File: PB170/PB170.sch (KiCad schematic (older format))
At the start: 50 parts, among them J1 USB_C_Receptacle_USB2.0-Conne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, J2 USB_B_Micro, Q1 P-MOSFET-MLP_HS, Q2 BC817, SW1 SW_MEC_5E, SW2 SW_MEC_5E

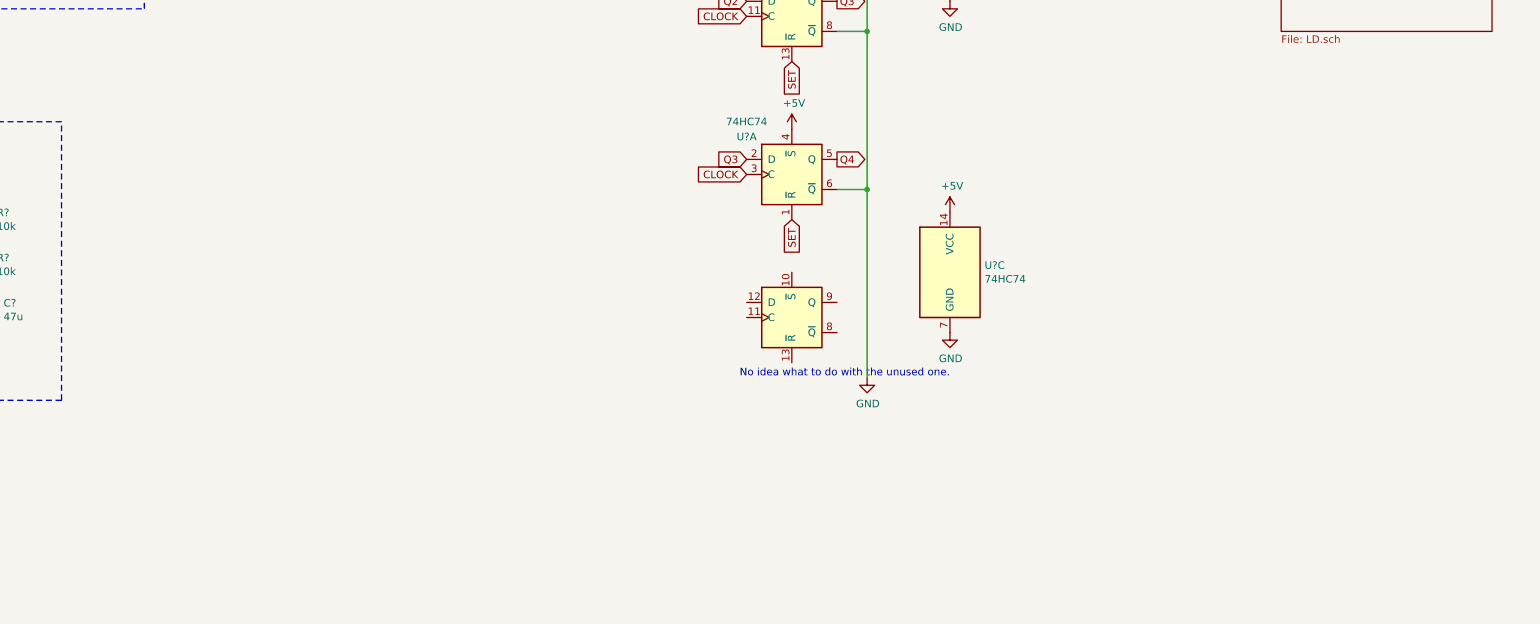
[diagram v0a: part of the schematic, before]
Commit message: PB170.sch change
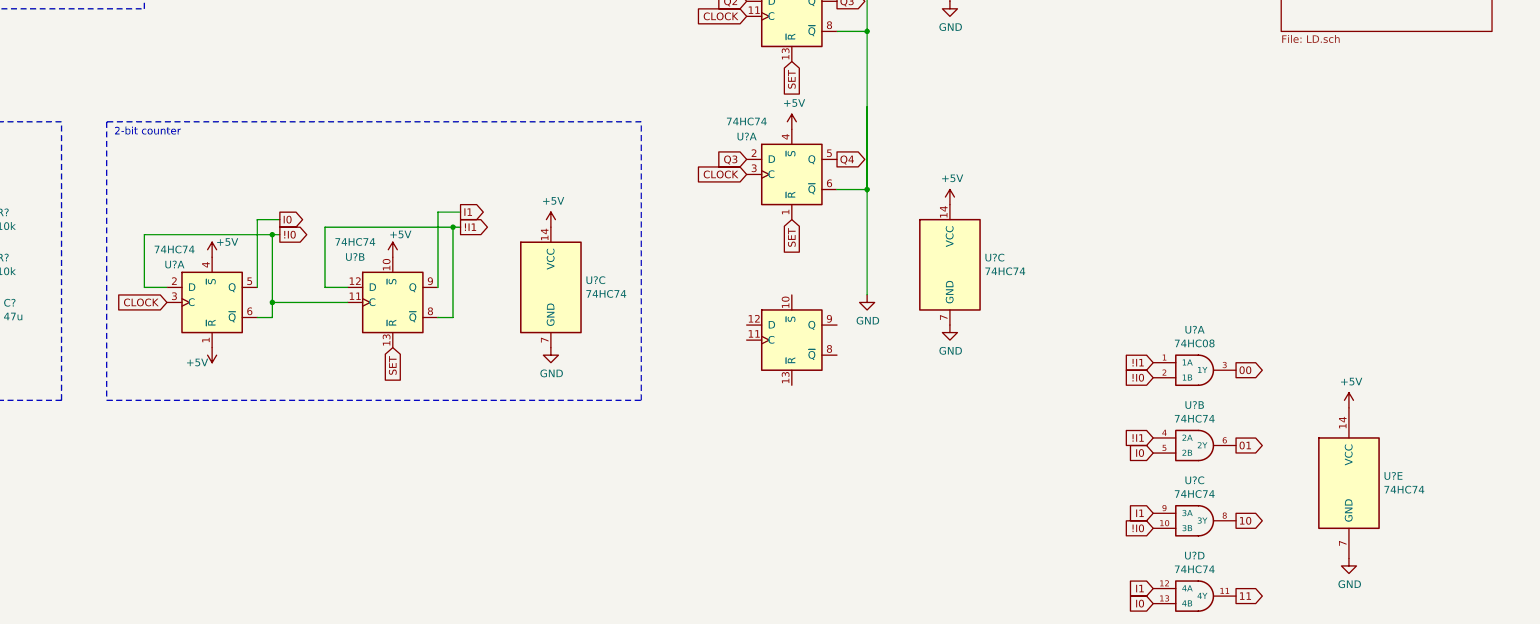
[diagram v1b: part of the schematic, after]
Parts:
- added U?: 74HC08, Housings_SOIC:SOIC-14_3.9x8.7mm_Pitch1.27mm, symbol PB170:74HC08
- added U? (x4): 74HC74, Package_SO:TSSOP-14_4.4x5mm_P0.65mm, symbol PB170:74HC08
- added U? (x3): 74HC74, Package_SO:TSSOP-14_4.4x5mm_P0.65mm, symbol 74xx:74HC74
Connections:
- net +5V: now also U?.1 (~R), U?.10 (~S), U?.14 (VCC), U?.14 (VCC), U?.4 (~S)
- net CLOCK: now also U?.3 (C)
- net GND: now also U?.7 (GND), U?.7 (GND)
- net SET: now also U?.13 (~R)
- new net !I0: U?.10 (3B), U?.11 (C), U?.2 (1B), U?.2 (D), U?.6 (~Q)
- new net !I1: U?.1 (1A), U?.12 (D), U?.4 (2A), U?.8 (~Q)
- new net 00: U?.3 (1Y)
- new net 01: U?.6 (2Y)
- new net 10: U?.8 (3Y)
- new net 11: U?.11 (4Y)
- new net I0: U?.13 (4B), U?.5 (2B), U?.5 (Q)
- new net I1: U?.12 (4A), U?.9 (3A), U?.9 (Q)
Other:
- note added: "2-bit counter"
- note removed: "No idea what to do with the unused one."
- moved on the sheet: U?C
